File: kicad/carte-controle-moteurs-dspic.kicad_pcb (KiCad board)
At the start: 4 copper layers, 142.2 x 81.3 mm, 72 parts, among them J1 PDB, J10 PWR_IN, J11 GND, J12 5V, J13 3.3V, J14 EN, J15 MOTEUR 1, J16 MOTEUR 2, J17 L1, J18 H1, J19 L2, J2 I2C, J20 H2, J21 ENCODEUR 1, J22 RA1, J23 ENCODEUR 2, J3 PROG, J4 PILES, J5 PILES, J6 Fix, J7 Fix, J8 Fix, J9 Fix, U1 L298_PAI225, U2 DSPIC33FJ, Y1 10MHz

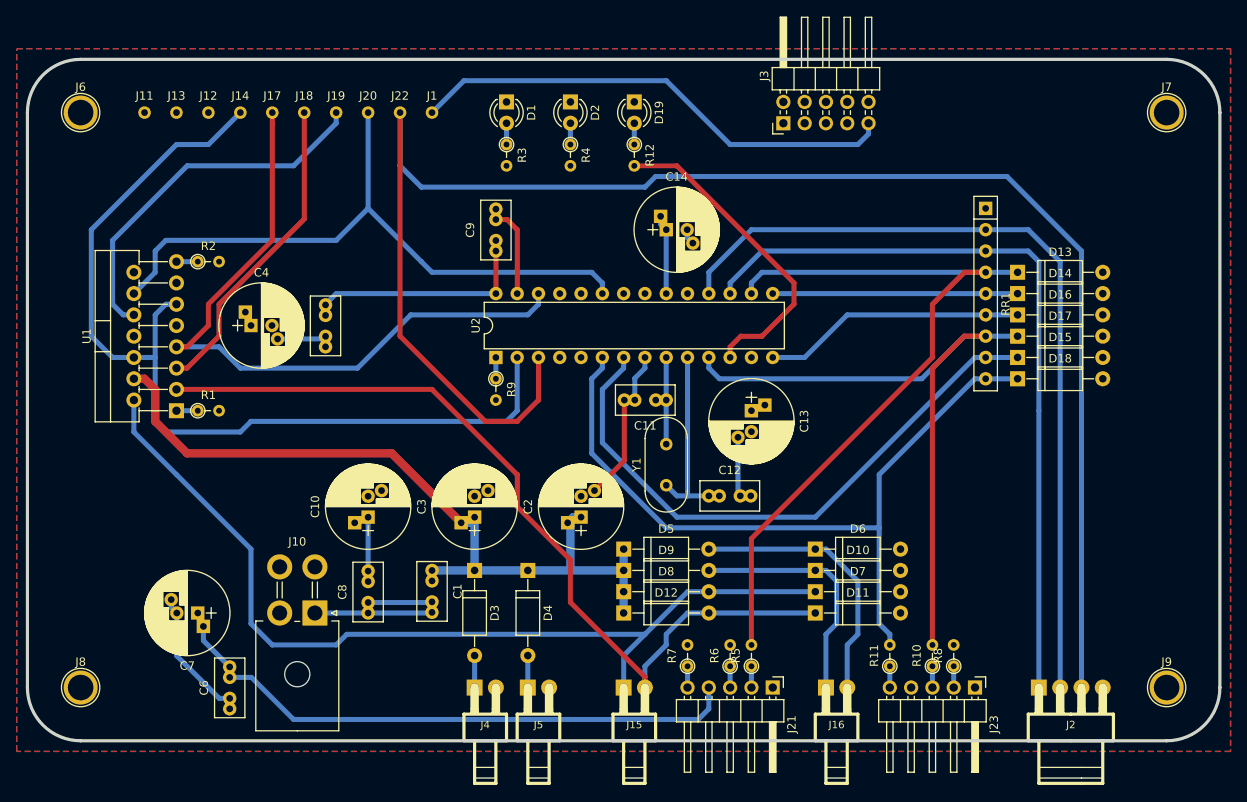
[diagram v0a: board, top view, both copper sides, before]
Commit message: Finalisation du typon
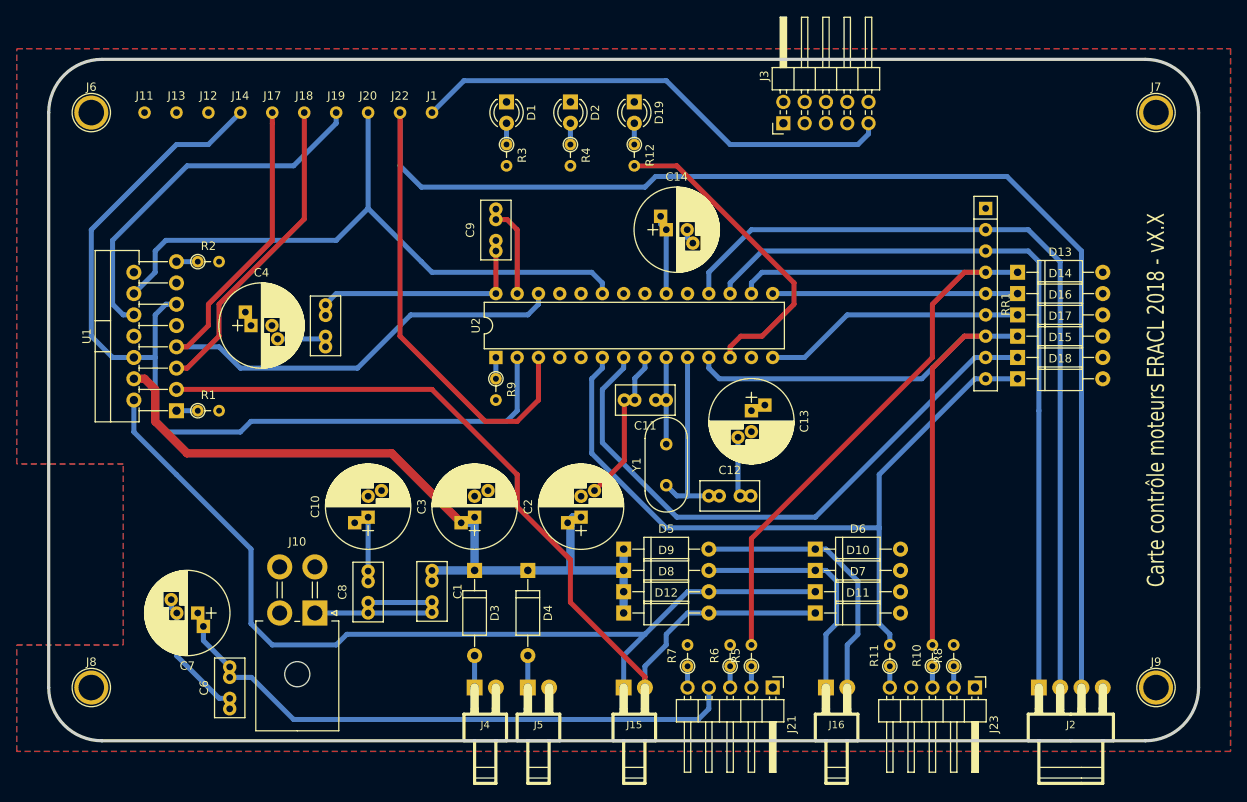
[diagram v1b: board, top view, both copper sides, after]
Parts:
- moved J6 1.27 mm to (29.2, 41.9)
- moved J8 1.27 mm to (29.2, 110.5)
- moved J7 1.27 mm to (156.2, 41.9)
- moved J9 1.27 mm to (156.2, 110.5)
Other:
- board size 142.2 x 81.3 mm -> 137.2 x 81.3 mm
- board text added: "Carte contrôle moteurs ERACL 2018 - vX.X"
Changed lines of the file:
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@@
     (links 170)
     (no_connects 0)
-    (area 6.35 24.13 165.100001 122.364501)
+    (area 20.32 29.800999 165.100001 122.364501)
     (thickness 1.6002)
-    (drawings 8)
+    (drawings 9)
     (tracks 340)
     (zones 0)
@@
     (2 Interne2 signal)
     (31 Dessous signal)
-    (32 B.Adhes user)
-    (33 F.Adhes user)
-    (34 B.Paste user)
-    (35 F.Paste user)
-    (36 B.SilkS user)
+    (32 B.Adhes user hide)
+    (33 F.Adhes user hide)
+    (34 B.Paste user hide)
+    (35 F.Paste user hide)
+    (36 B.SilkS user hide)
     (37 F.SilkS user)
     (38 B.Mask user)
     (39 F.Mask user)
-    (40 Dwgs.User user)
-    (41 Cmts.User user)
-    (42 Eco1.User user)
-    (43 Eco2.User user)
+    (40 Dwgs.User user hide)
+    (41 Cmts.User user hide)
+    (42 Eco1.User user hide)
+    (43 Eco2.User user hide)
     (44 Edge.Cuts user)
   )
@@
     (pad_to_mask_clearance 0.254)
     (aux_axis_origin 0 0)
-    (visible_elements FFFFFFFF)
+    (visible_elements FFFFF73F)
     (pcbplotparams
       (layerselection 0x00030_80000001)
@@
   )
   (module Connectors:1pin (layer Dessus)
-    (at 27.94 41.91)
+    (at 29.21 41.91)
     (descr "module 1 pin (ou trou mecanique de percage)")
     (tags DEV)
@@
   )
   (module Connectors:1pin (layer Dessus)
-    (at 157.48 41.91)
+    (at 156.21 41.91)
     (descr "module 1 pin (ou trou mecanique de percage)")
     (tags DEV)
@@
   )
   (module Connectors:1pin (layer Dessus)
-    (at 27.94 110.49)
+    (at 29.21 110.49)
     (descr "module 1 pin (ou trou mecanique de percage)")
     (tags DEV)
@@
   )
   (module Connectors:1pin (layer Dessus)
-    (at 157.48 110.49)
+    (at 156.21 110.49)
     (descr "module 1 pin (ou trou mecanique de percage)")
     (tags DEV)
@@
     )
   )
-  (gr_line (start 157.48 35.56) (end 27.94 35.56) (angle 90) (layer Edge.Cuts) (width 0.381))
-  (gr_line (start 163.83 110.49) (end 163.83 41.91) (angle 90) (layer Edge.Cuts) (width 0.381))
-  (gr_line (start 27.94 116.84) (end 157.48 116.84) (angle 90) (layer Edge.Cuts) (width 0.381))
-  (gr_line (start 21.59 41.91) (end 21.59 110.49) (angle 90) (layer Edge.Cuts) (width 0.381))
-  (gr_arc (start 27.94 41.91) (end 21.59 41.91) (angle 90) (layer Edge.Cuts) (width 0.381))
-  (gr_arc (start 157.48 41.91) (end 157.48 35.56) (angle 90) (layer Edge.Cuts) (width 0.381))
-  (gr_arc (start 27.94 110.49) (end 27.94 116.84) (angle 90) (layer Edge.Cuts) (width 0.381))
-  (gr_arc (start 157.48 110.49) (end 163.83 110.49) (angle 90) (layer Edge.Cuts) (width 0.381))
+  (gr_text "Carte contrôle moteurs ERACL 2018 - vX.X" (at 156.21 76.2 90) (layer F.SilkS)
+    (effects (font (size 2.032 1.524) (thickness 0.3048)))
+  )
+  (gr_line (start 154.94 116.84) (end 30.48 116.84) (angle 90) (layer Edge.Cuts) (width 0.381))
+  (gr_line (start 30.48 35.56) (end 154.94 35.56) (angle 90) (layer Edge.Cuts) (width 0.381))
+  (gr_line (start 161.29 110.49) (end 161.29 41.91) (angle 90) (layer Edge.Cuts) (width 0.381))
+  (gr_line (start 24.13 41.91) (end 24.13 110.49) (angle 90) (layer Edge.Cuts) (width 0.381))
+  (gr_arc (start 30.48 41.91) (end 24.13 41.91) (angle 90) (layer Edge.Cuts) (width 0.381))
+  (gr_arc (start 154.94 41.91) (end 154.94 35.56) (angle 90) (layer Edge.Cuts) (width 0.381))
+  (gr_arc (start 30.48 110.49) (end 30.48 116.84) (angle 90) (layer Edge.Cuts) (width 0.381))
+  (gr_arc (start 154.94 110.49) (end 161.29 110.49) (angle 90) (layer Edge.Cuts) (width 0.381))
   (segment (start 45.72 109.28) (end 48.32 109.28) (width 0.59944) (layer Dessous) (net 1))
   (segment (start 102.87 113.03) (end 102.87 110.49) (width 0.59944) (layer Dessous) (net 1))
@@
     (polygon
       (pts
-        (xy 165.1 118.11) (xy 20.32 118.11) (xy 20.32 34.29) (xy 165.1 34.29)
+        (xy 165.1 118.11) (xy 20.32 118.11) (xy 20.32 105.41) (xy 33.02 105.41) (xy 33.02 83.82)
+        (xy 20.32 83.82) (xy 20.32 34.29) (xy 165.1 34.29)
       )
     )
@@
     (polygon
       (pts
-        (xy 165.1 118.11) (xy 20.32 118.11) (xy 20.32 34.29) (xy 165.1 34.29)
+        (xy 165.1 118.11) (xy 20.32 118.11) (xy 20.32 105.41) (xy 33.02 105.41) (xy 33.02 83.82)
+        (xy 20.32 83.82) (xy 20.32 34.29) (xy 165.1 34.29)
       )
     )
@@
     (polygon
       (pts
-        (xy 165.1 118.11) (xy 20.32 118.11) (xy 20.32 34.29) (xy 165.1 34.29)
+        (xy 165.1 118.11) (xy 20.32 118.11) (xy 20.32 105.41) (xy 33.02 105.41) (xy 33.02 83.82)
+        (xy 20.32 83.82) (xy 20.32 34.29) (xy 165.1 34.29)
       )
     )
@@
     (polygon
       (pts
-        (xy 165.1 118.11) (xy 20.32 118.11) (xy 20.32 34.29) (xy 165.1 34.29)
+        (xy 165.1 118.11) (xy 20.32 118.11) (xy 20.32 105.41) (xy 33.02 105.41) (xy 33.02 83.82)
+        (xy 20.32 83.82) (xy 20.32 34.29) (xy 165.1 34.29)
       )
     )
